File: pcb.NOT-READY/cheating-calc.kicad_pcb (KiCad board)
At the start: 2 copper layers, 72 x 22 mm, 22 parts, among them J1 Conn_01x04, J2 Conn_01x04, Q1 MMBF170, Q2 MMBF170, U1 ESP32-C3-MINI-1-N4, U2 AP7215-33YG-13

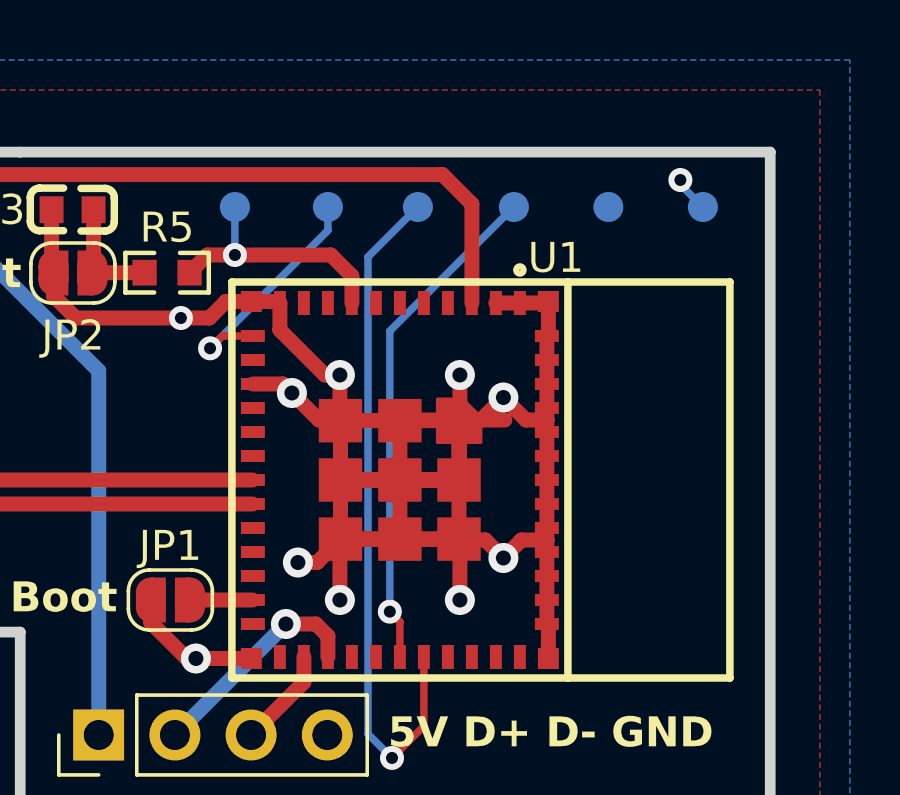
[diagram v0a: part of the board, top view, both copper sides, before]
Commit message: update
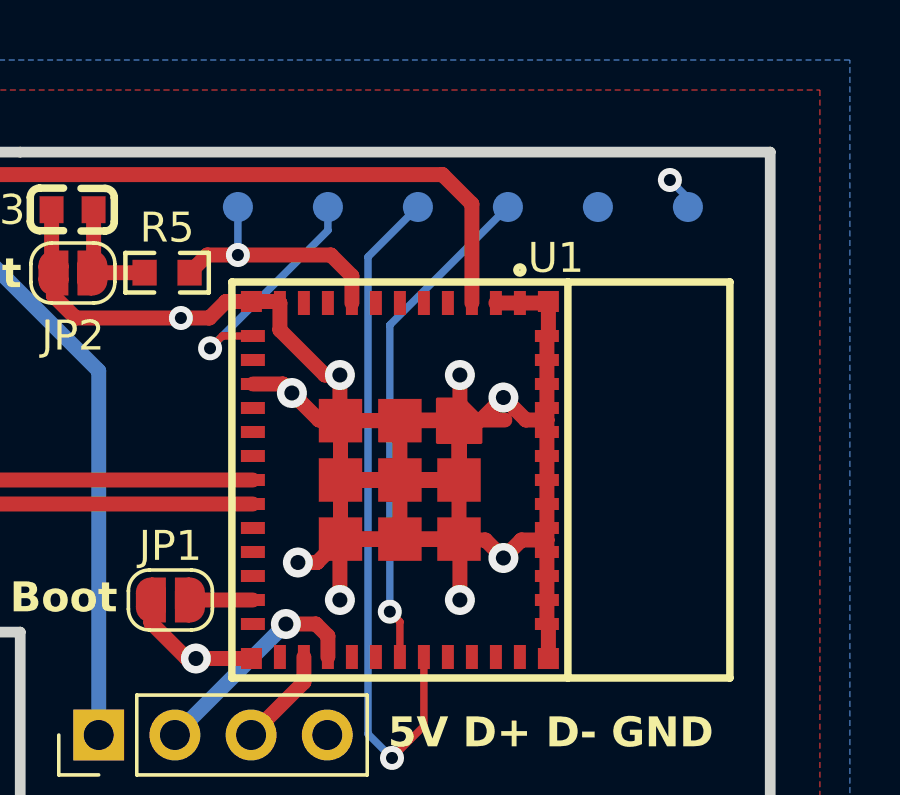
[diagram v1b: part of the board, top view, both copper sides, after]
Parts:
- moved TP1 0.50 mm to (154.6, 53.9)
- moved TP2 0.35 mm to (151.6, 53.9)
- moved TP3 0.20 mm to (148.6, 53.9)
- moved TP6 0.10 mm to (139.6, 53.9)
